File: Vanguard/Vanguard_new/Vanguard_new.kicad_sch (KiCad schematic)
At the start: 72 parts, among them J1 USB_C, J2 Conn_02x03_Pin, J3 Micro_SD_Card_Det1, J4 STARBOARD_SERVO, J5 PORTSIDE_SERVO, J6 Conn_01x02_Pin, Q1 BSS138, Q2 BSS138, Q3 BSS138, Q4 BSS138, U1 ATSAMD11D14A-M, U2 ATmega4809-A, U3 AT25DF641A-SH-T, U4 AP2112K-3.3, U5 MPM3610AGQV-P, U6 BNO086, U7 TXB0104D, U8 TPS61092, Y1 32.768kHz

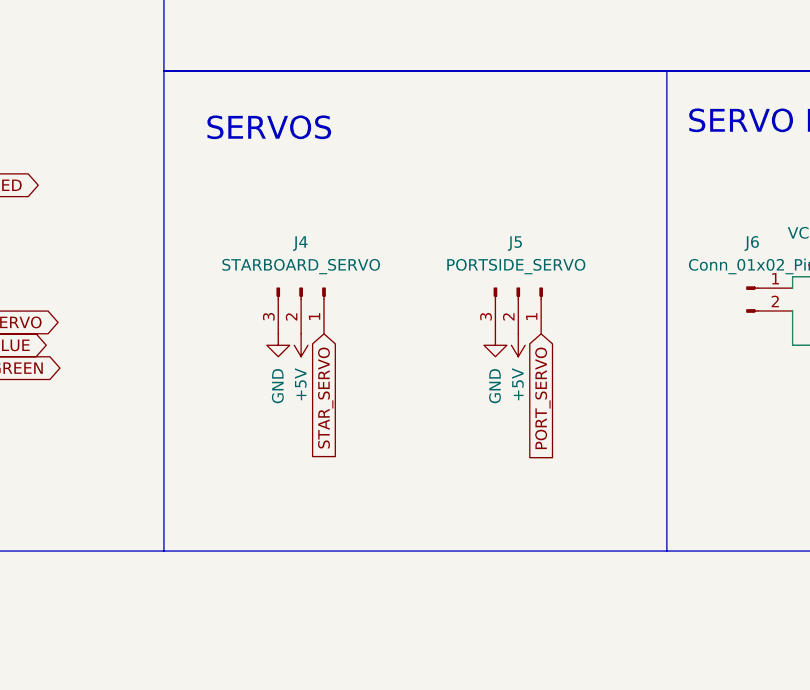
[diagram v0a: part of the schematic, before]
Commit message: fixed many errors
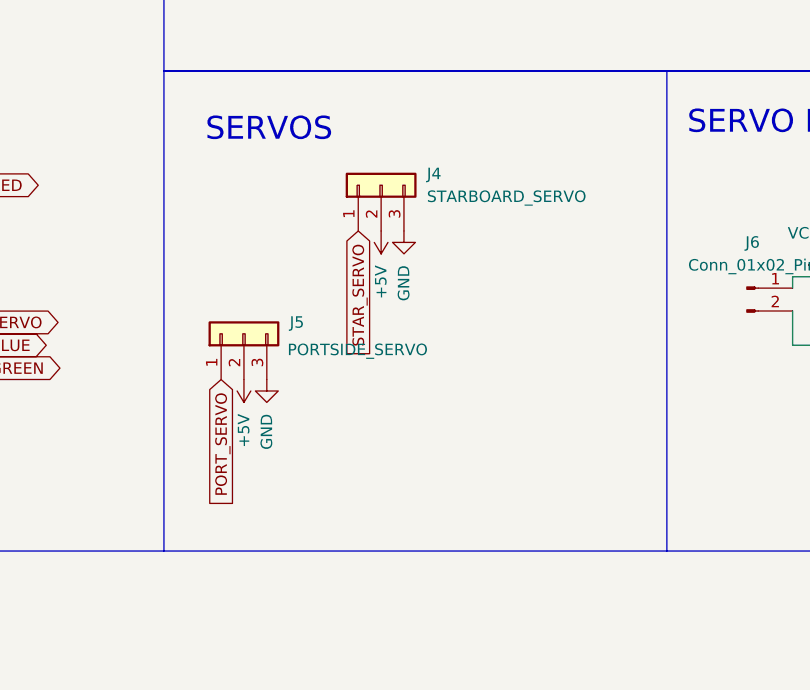
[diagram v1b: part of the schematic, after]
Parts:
- removed J4: STARBOARD_SERVO, Connector_PinHeader_2.54mm:PinHeader_1x03_P2.54mm_Vertical, symbol Connector:Conn_01x03_Pin
- removed J5: PORTSIDE_SERVO, Connector_PinHeader_2.54mm:PinHeader_1x03_P2.54mm_Vertical, symbol Connector:Conn_01x03_Pin
- added J4: STARBOARD_SERVO, Connector_PinHeader_2.54mm:PinHeader_1x03_P2.54mm_Vertical, symbol Connector_Generic:Conn_01x03
- added J5: PORTSIDE_SERVO, Connector_PinHeader_2.54mm:PinHeader_1x03_P2.54mm_Vertical, symbol Connector_Generic:Conn_01x03
- U8: footprint Package_DFN_QFN:Texas_RSA_VQFN-16-1EP_4x4mm_P0.65mm_EP2.7x2.7mm_ThermalVias -> Package_DFN_QFN:DFN-10-1EP_3x3mm_P0.5mm_EP1.65x2.38mm_ThermalVias
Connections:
- net +5V: now also J4.2 (Pin_2), J5.2 (Pin_2)
- net GND: now also J4.3 (Pin_3), J5.3 (Pin_3)
- net PORT_SERVO: now also J5.1 (Pin_1)
- net STAR_SERVO: now also J4.1 (Pin_1)
